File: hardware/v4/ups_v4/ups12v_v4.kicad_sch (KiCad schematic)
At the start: 61 parts, among them IC1 BQ25798RQMR, J1 ADAPTER 4.75-21V, J2 VSYS OUTPUT, J3 BATTERY 2S/4S, J4 MCU / BIAS INTERFACE, J6 NTC temp sensor, Q1 AON7528, Q2 AON7528, Q3 PMV16UN

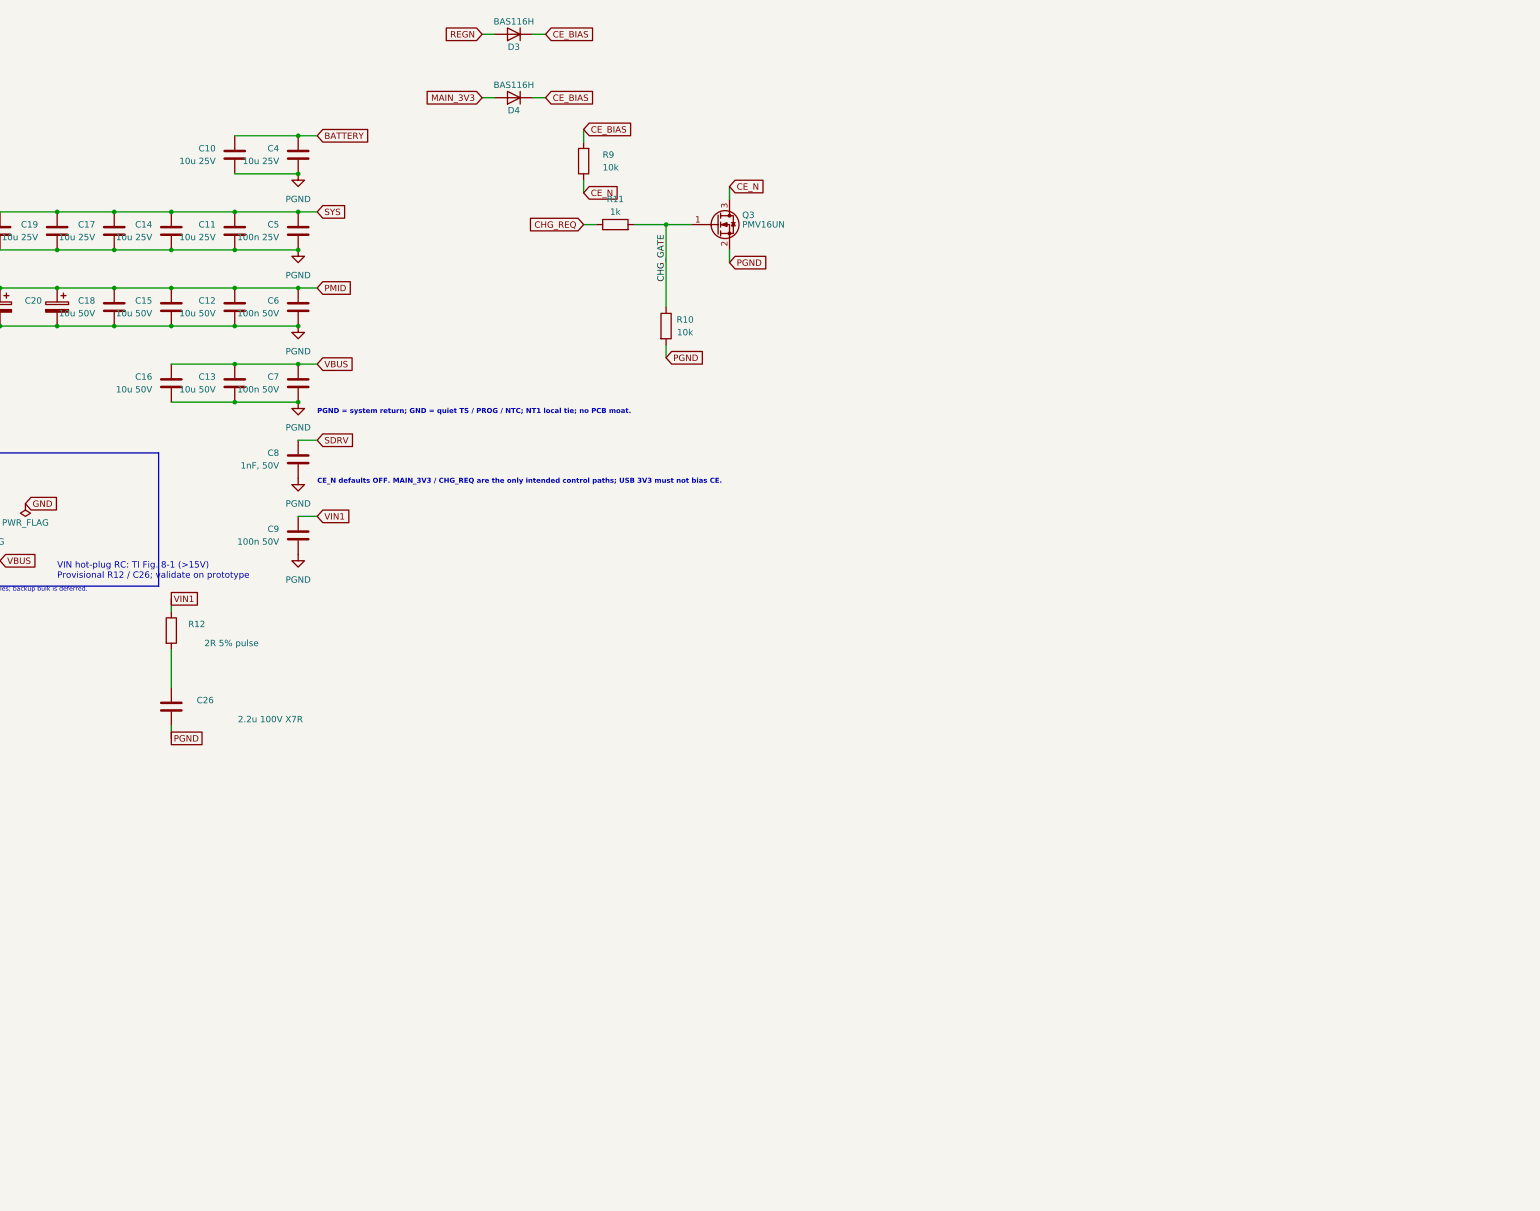
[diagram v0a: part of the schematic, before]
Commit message: phase 3.1
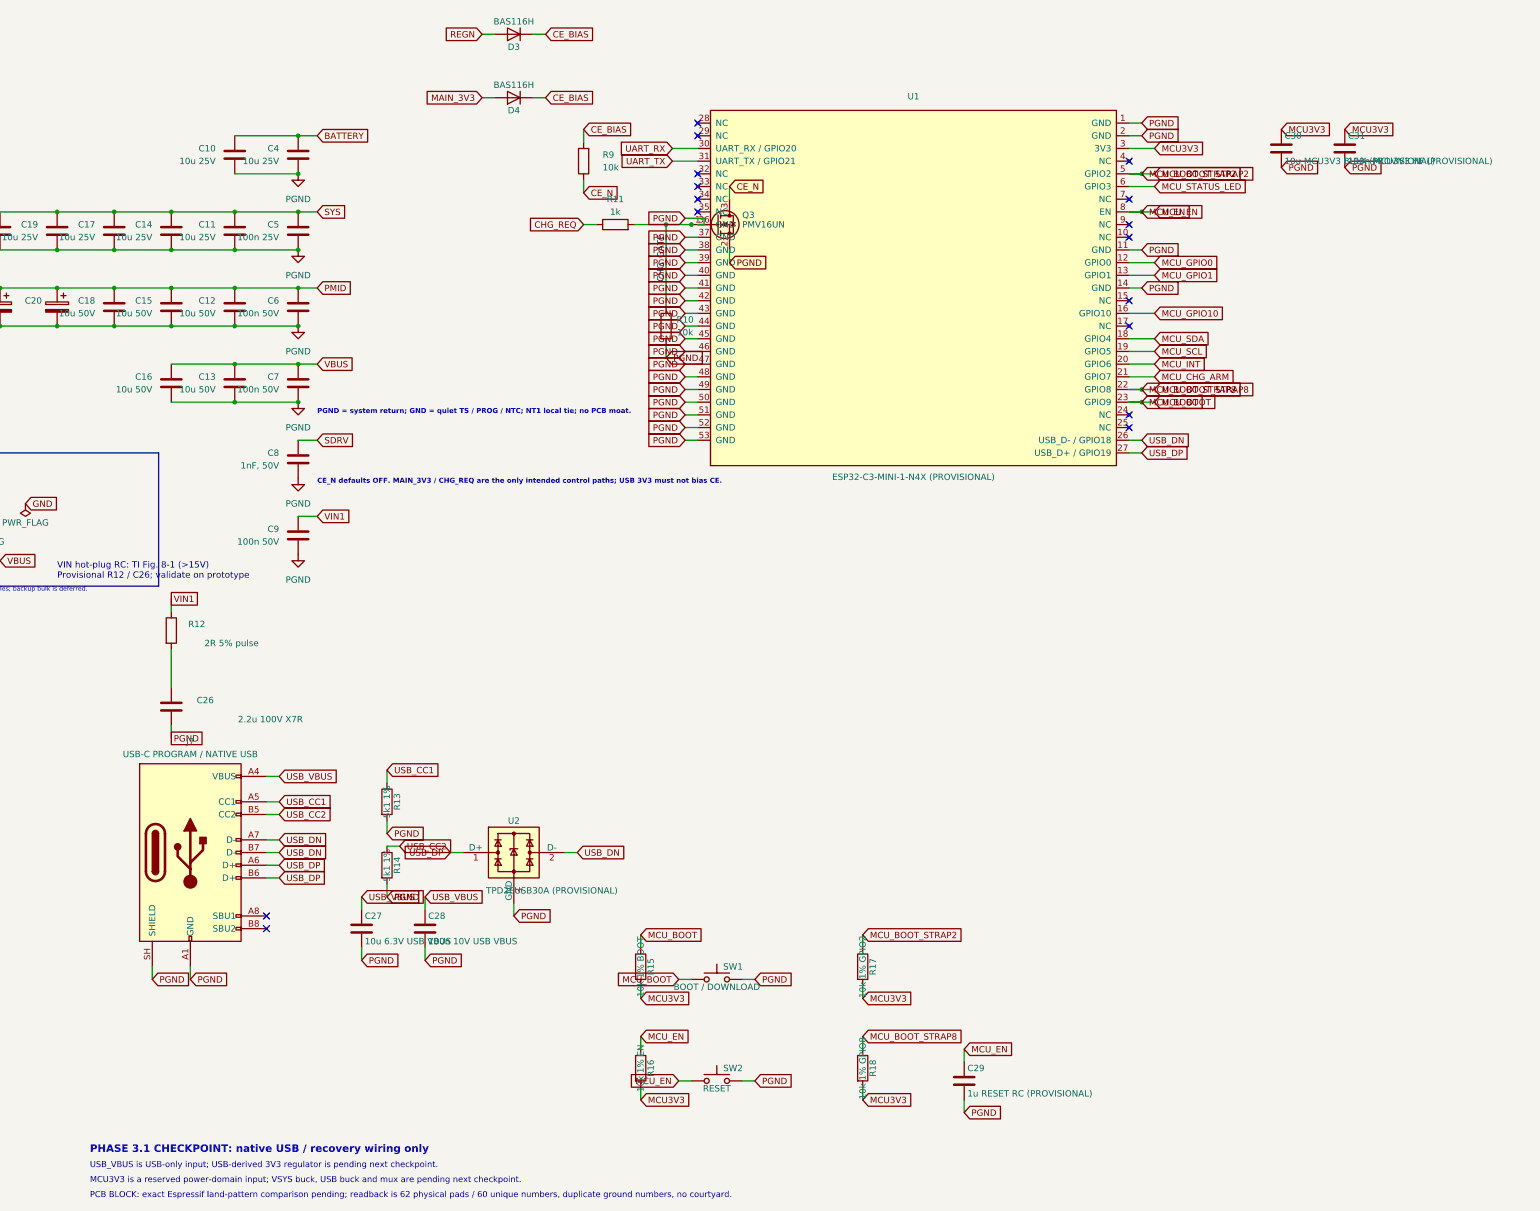
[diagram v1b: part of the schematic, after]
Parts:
- added C27: 10u 6.3V USB VBUS, Capacitor_SMD:C_0805_2012Metric, symbol Device:C
- added C28: 100n 10V USB VBUS, Capacitor_SMD:C_0402_1005Metric, symbol Device:C
- added C29: 1u RESET RC (PROVISIONAL), Capacitor_SMD:C_0402_1005Metric, symbol Device:C
- added C30: 10u MCU3V3 BULK (PROVISIONAL), Capacitor_SMD:C_0805_2012Metric, symbol Device:C
- added C31: 100n MCU3V3 HF (PROVISIONAL), Capacitor_SMD:C_0402_1005Metric, symbol Device:C
- added J7: USB-C PROGRAM / NATIVE USB, Connector_USB:USB_C_Receptacle_GCT_USB4105-xx-A_16P_TopMnt_Horizontal, symbol Connector:USB_C_Receptacle_USB2.0_16P
- added R13, R14: 5k1 1%, Resistor_SMD:R_0402_1005Metric, symbol Device:R
- added R15: 10k 1% BOOT, Resistor_SMD:R_0402_1005Metric, symbol Device:R
- added R16: 10k 1% EN, Resistor_SMD:R_0402_1005Metric, symbol Device:R
- added R17: 10k 1% GPIO2, Resistor_SMD:R_0402_1005Metric, symbol Device:R
- added R18: 10k 1% GPIO8, Resistor_SMD:R_0402_1005Metric, symbol Device:R
- added SW1: BOOT / DOWNLOAD, Button_Switch_SMD:SW_SPST_EVQP0, symbol Switch:SW_Push
- added SW2: RESET, Button_Switch_SMD:SW_SPST_EVQP0, symbol Switch:SW_Push
- added U1: ESP32-C3-MINI-1-N4X (PROVISIONAL), Modules_MCU:ESP32-C3-MINI-1, symbol ups_v4_custom:ESP32-C3-MINI-1
- added U2: TPD2EUSB30A (PROVISIONAL), Package_TO_SOT_SMD:SOT-23, symbol Power_Protection:TPD2EUSB30A
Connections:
- net PGND: now also C27.2, C28.2, C29.2, C30.2, C31.2, J7.A1 (GND), J7.A12 (GND), J7.B1 (GND), J7.B12 (GND), J7.SH (SHIELD), R13.2, R14.2, SW1.2, SW2.2, U1.1 (GND), U1.11 (GND), U1.14 (GND), U1.2 (GND), U1.36 (GND), U1.37 (GND), U1.38 (GND), U1.39 (GND), U1.40 (GND), U1.41 (GND), U1.42 (GND), U1.43 (GND), U1.44 (GND), U1.45 (GND), U1.46 (GND), U1.47 (GND), U1.48 (GND), U1.49 (GND), U1.50 (GND), U1.51 (GND), U1.52 (GND), U1.53 (GND), U2.3 (GND)
- new net MCU3V3: C30.1, C31.1, R15.2, R16.2, R17.2, R18.2, U1.3 (3V3)
- new net MCU_BOOT: R15.1, SW1.1, U1.23 (GPIO9)
- new net MCU_BOOT_STRAP2: R17.1, U1.5 (GPIO2)
- new net MCU_BOOT_STRAP8: R18.1, U1.22 (GPIO8)
- new net MCU_CHG_ARM: U1.21 (GPIO7)
- new net MCU_EN: C29.1, R16.1, SW2.1, U1.8 (EN)
- new net MCU_GPIO0: U1.12 (GPIO0)
- new net MCU_GPIO1: U1.13 (GPIO1)
- new net MCU_GPIO10: U1.16 (GPIO10)
- new net MCU_INT: U1.20 (GPIO6)
- new net MCU_SCL: U1.19 (GPIO5)
- new net MCU_SDA: U1.18 (GPIO4)
- new net MCU_STATUS_LED: U1.6 (GPIO3)
- new net UART_RX: U1.30 (UART_RX / GPIO20)
- new net UART_TX: U1.31 (UART_TX / GPIO21)
- new net USB_CC1: J7.A5 (CC1), R13.1
- new net USB_CC2: J7.B5 (CC2), R14.1
- new net USB_DN: J7.A7 (D-), J7.B7 (D-), U1.26 (USB_D- / GPIO18), U2.2 (D-)
- new net USB_DP: J7.A6 (D+), J7.B6 (D+), U1.27 (USB_D+ / GPIO19), U2.1 (D+)
- new net USB_VBUS: C27.1, C28.1, J7.A4 (VBUS), J7.A9 (VBUS), J7.B4 (VBUS), J7.B9 (VBUS)
- no-connect marks 3 -> 19
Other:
- note added: "MCU3V3 is a reserved power-domain input; VSYS buck, USB buck and mux are pending next checkpoint."
- note added: "PCB BLOCK: exact Espressif land-pattern comparison pending; readback is 62 physical pads / 60 unique numbers, duplicate ground numbers, no courtyard."
- note added: "PHASE 3.1 CHECKPOINT: native USB / recovery wiring only"
- note added: "USB_VBUS is USB-only input; USB-derived 3V3 regulator is pending next checkpoint."
